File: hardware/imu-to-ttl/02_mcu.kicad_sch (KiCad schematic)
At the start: 6 parts, among them J2 SWD+UART+NRST, U1 STM32G031F8P6

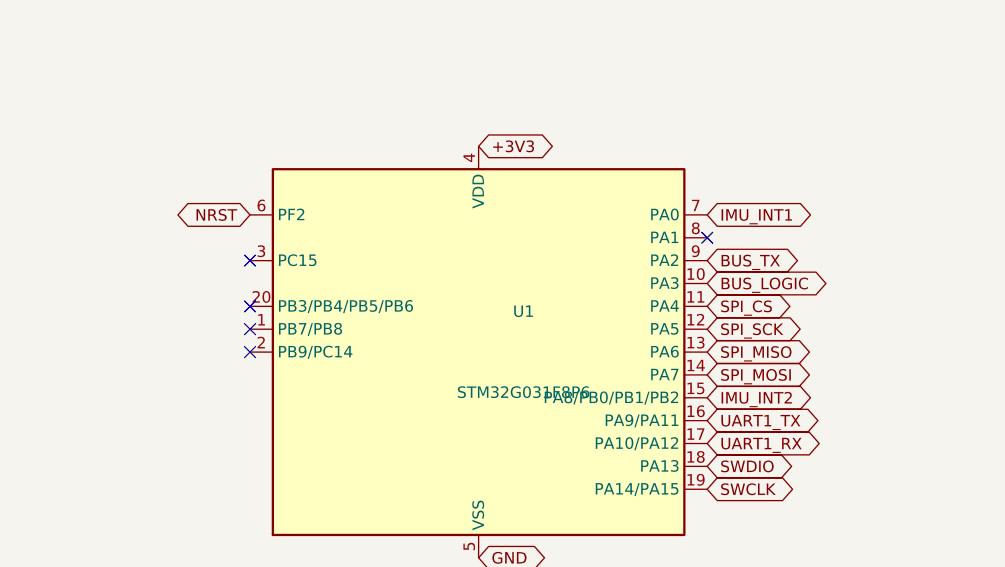
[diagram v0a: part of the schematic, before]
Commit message: sync: 2026-10-12 日常更新
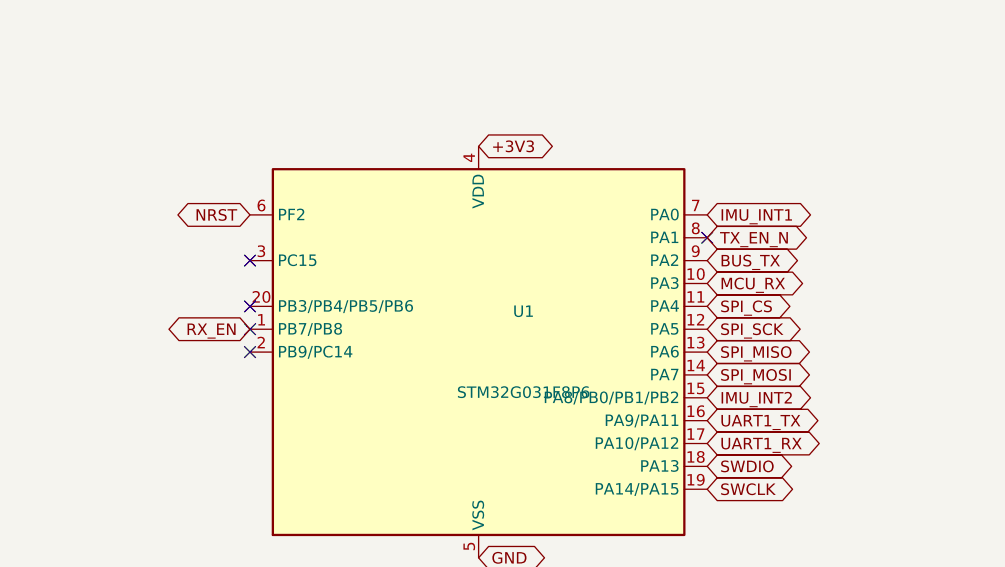
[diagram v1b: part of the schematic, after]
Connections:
- net RX_EN: now reaches U1.1 (PB7/PB8)
- net TX_EN_N: now reaches U1.8 (PA1)
- net BUS_LOGIC renamed MCU_RX
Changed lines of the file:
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@@
 	)
+	)
+	(global_label "TX_EN_N"
+		(shape bidirectional)
+		(at 125.73 97.79 0)
+		(fields_autoplaced yes)
+		(effects
+			(font
+				(size 1.27 1.27)
+			)
+			(justify left)
+		)
+		(property "Intersheetrefs" "${INTERSHEET_REFS}"
+			(at 125.73 97.79 0)
+			(effects
+				(font
+					(size 1.27 1.27)
+				)
+				(hide yes)
+			)
+		)
+	)
+	(global_label "RX_EN"
+		(shape bidirectional)
+		(at 74.93 107.95 180)
+		(fields_autoplaced yes)
+		(effects
+			(font
+				(size 1.27 1.27)
+			)
+			(justify right)
+		)
+		(property "Intersheetrefs" "${INTERSHEET_REFS}"
+			(at 74.93 107.95 0)
+			(effects
+				(font
+					(size 1.27 1.27)
+				)
+				(hide yes)
+			)
+		)
 	)
 	(global_label "BUS_TX"
@@
 	)
 	)
-	(global_label "BUS_LOGIC"
+	(global_label "MCU_RX"
 		(shape bidirectional)
 		(at 125.73 102.87 0)
